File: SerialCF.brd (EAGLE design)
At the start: 101.6 x 34 mm, 4 parts, among them IC1 Z80CPU

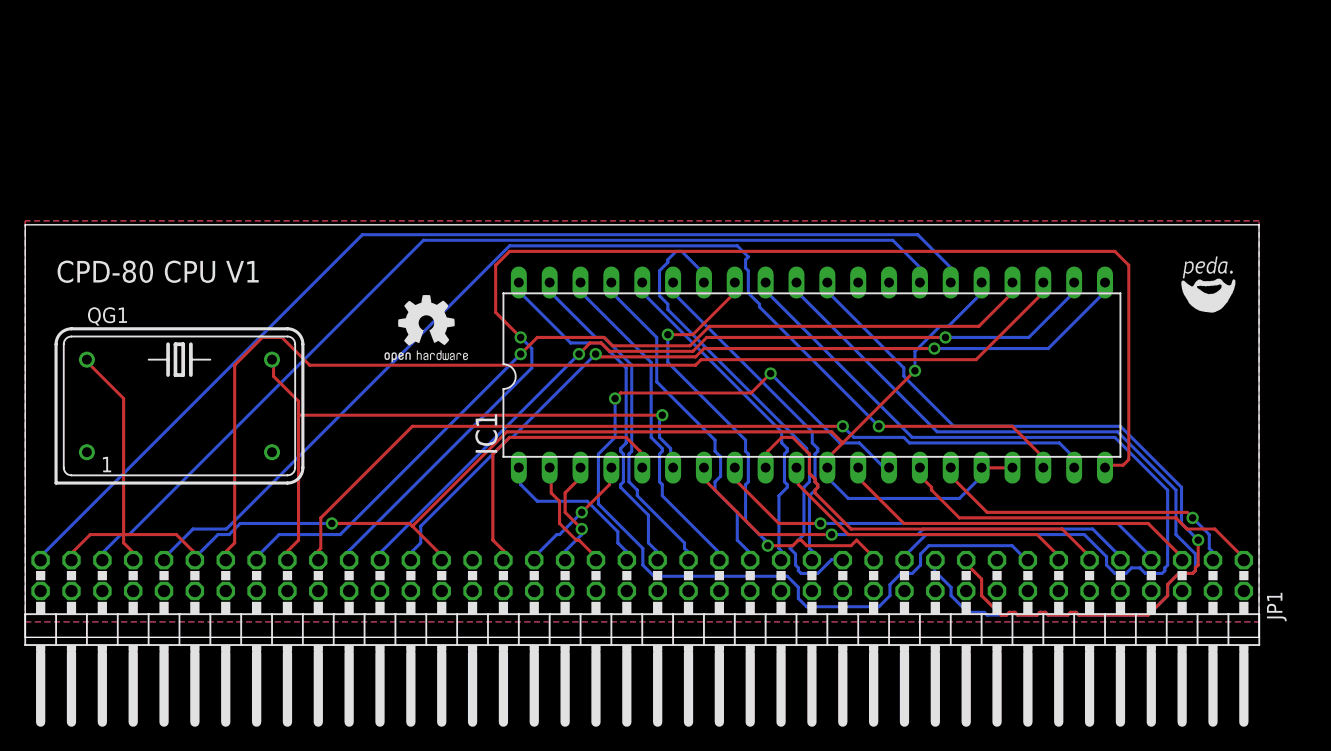
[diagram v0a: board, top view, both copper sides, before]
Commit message: Finish Modularization
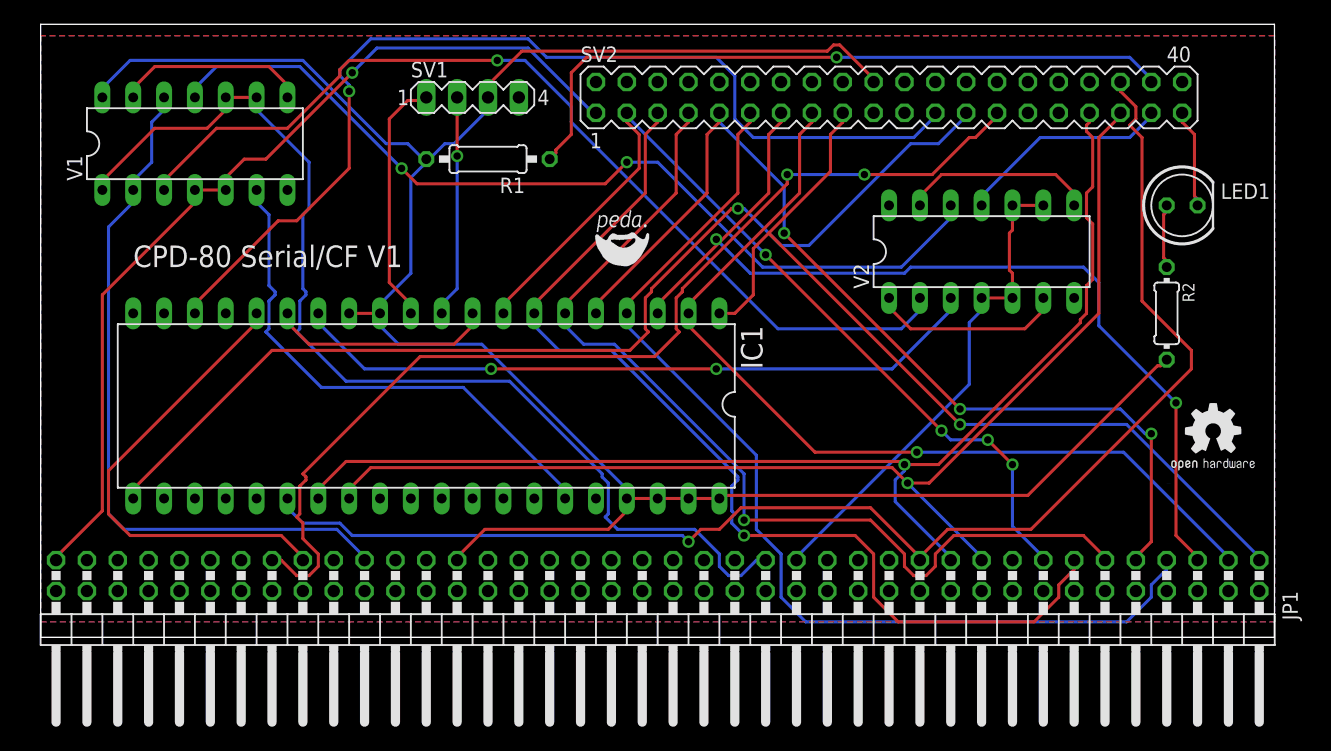
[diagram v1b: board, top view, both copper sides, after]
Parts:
- removed QG1: 6 MHz, crystal:DIL14S
- added LED1: AC, led:LED5MM
- added R1: 1k, eagle-ltspice:0207/10
- added R2: 560, resistor:0204/7
- added SV1: SERIAL, con-lstb:MA04-1
- added SV2: IDE PATA CF Card, con-lstb:MA20-2
- added V1, V2: 74HC00N, 74ttl-din:DIL14
- IC1: value Z80CPU -> XR-16C550P; device zilog:DIL40 -> exar:DIL40
- moved U$1 65.4 mm to (95.2, 12.7)
- moved IC1 31.9 mm to (34.3, 19.1), turned to 180 degrees
- moved JP1 1.27 mm to (73.7, 0.00)
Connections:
- removed net CLOCK: IC1.6, JP1.63, QG1.8
- removed net N$10: IC1.22, JP1.57
- removed net N$14: IC1.21, JP1.55
- removed net N$16: IC1.20, JP1.59
- removed net N$22: IC1.23, JP1.67
- removed net N$8: IC1.19, JP1.61
- removed net N$9: IC1.18, JP1.71
- new net !RD: IC1.21, SV2.25
- new net !WR: IC1.18, SV2.23
- new net +UB: V2.14
- new net -UB: V2.7
- new net IOCS1: SV2.37, V2.11
- new net N$11: IC1.11, SV1.1
- new net N$13: IC1.15, IC1.9
- new net N$15: IC1.10, SV1.2
- new net N$17: V1.13, V1.8
- new net N$18: IC1.14, V2.3
- new net N$19: JP1.59, V1.12, V1.2
- new net N$2: LED1.K, SV2.39
- new net N$20: R1.1, SV2.38
- new net N$3: LED1.A, R2.1
- new net N$4: V1.3, V2.2
- new net N$5: V2.1, V2.6
- new net N$6: V2.13, V2.8
- new net N$7: V1.11, V2.12
- new net RESET: IC1.35, V1.6
- net !RESET: now also SV2.1, V1.4, V1.5; no longer IC1.26
- net A0: now also IC1.28, SV2.35; no longer IC1.30
- net A1: now also IC1.27, SV2.33; no longer IC1.31
- net A10: no longer IC1.40
- net A11: no longer IC1.1
- net A12: no longer IC1.2
- net A13: no longer IC1.3
- net A14: no longer IC1.4
- net A15: no longer IC1.5
- net A2: now also IC1.26, SV2.36; no longer IC1.32
- net A3: no longer IC1.33
- net A4: no longer IC1.34
- net A5: no longer IC1.35
- net A6: now also V2.10, V2.4, V2.5, V2.9; no longer IC1.36
- net A7: now also V1.1, V1.10, V1.9; no longer IC1.37
- net A8: no longer IC1.38
- net A9: no longer IC1.39
- net D0: now also IC1.1, SV2.17; no longer IC1.14
- net D1: now also IC1.2, SV2.15; no longer IC1.15
- net D2: now also IC1.3, SV2.13; no longer IC1.12
- net D3: now also IC1.4, SV2.11; no longer IC1.8
- net D4: now also IC1.5, SV2.9; no longer IC1.7
- net D5: now also IC1.6, SV2.7; no longer IC1.9
- net D6: now also IC1.7, SV2.5; no longer IC1.10
- net D7: now also IC1.8, SV2.3; no longer IC1.13
- net GND: now also IC1.19, IC1.20, IC1.22, IC1.25, SV1.4, SV2.19, SV2.2, SV2.22, SV2.24, SV2.26, SV2.30, SV2.40, V1.7; no longer IC1.29, QG1.7
- net N$1: now also IC1.16, JP1.63; no longer IC1.27, JP1.75
- net VCC: now also IC1.12, IC1.13, IC1.37, IC1.38, IC1.39, IC1.40, R1.2, R2.2, SV1.3, SV2.20, V1.14; no longer IC1.11, IC1.16, IC1.17, IC1.25, JP1.69, JP1.73, JP1.77, QG1.14
- net WAIT: now also SV2.27; no longer IC1.24
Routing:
- net N$16: track 103.1 -> 0.00 mm, vias 1 -> 0
- net N$9: track 93.5 -> 0.00 mm, vias 1 -> 0
- net N$22: track 88.1 -> 0.00 mm
- net !RD: track 0.00 -> 87.0 mm, vias 0 -> 1
- net !WR: track 0.00 -> 83.0 mm, vias 0 -> 1
- net N$4: track 0.00 -> 78.9 mm, vias 0 -> 1
- net N$7: track 0.00 -> 74.7 mm, vias 0 -> 2
- net N$8: track 70.6 -> 0.00 mm, vias 1 -> 0
- net N$14: track 68.4 -> 0.00 mm, vias 2 -> 0
- net N$10: track 68.0 -> 0.00 mm, vias 2 -> 0
- net A7: track 28.0 -> 88.8 mm
- net N$19: track 0.00 -> 59.0 mm
- net D6: track 25.8 -> 84.7 mm, vias 0 -> 1
- net N$18: track 0.00 -> 57.4 mm, vias 0 -> 2
- net N$20: track 0.00 -> 57.1 mm, vias 0 -> 1
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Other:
- board size 101.6 x 34 mm -> 101.6 x 50.5 mm
- board text added: "+"
- board text added: "-"
- board text added: "CPD-80 Serial/CF V1"
- board text added: "RX"
- board text added: "TX"
- board text removed: "CPD-80 CPU V1"
